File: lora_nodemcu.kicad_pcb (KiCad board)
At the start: 4 copper layers, 33 x 39.4 mm, 9 parts, among them U1 RFM95, U3 WeMos_mini

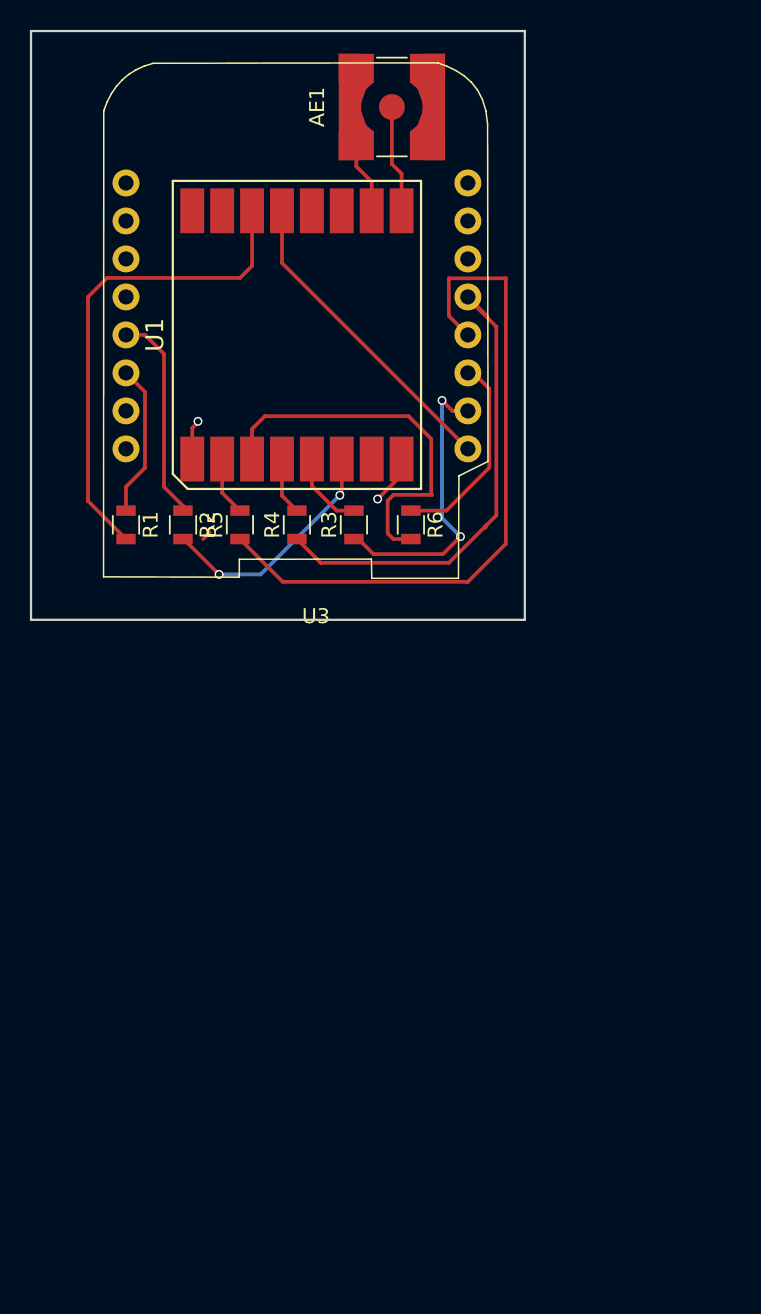
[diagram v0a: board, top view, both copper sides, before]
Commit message: Relayed out board.
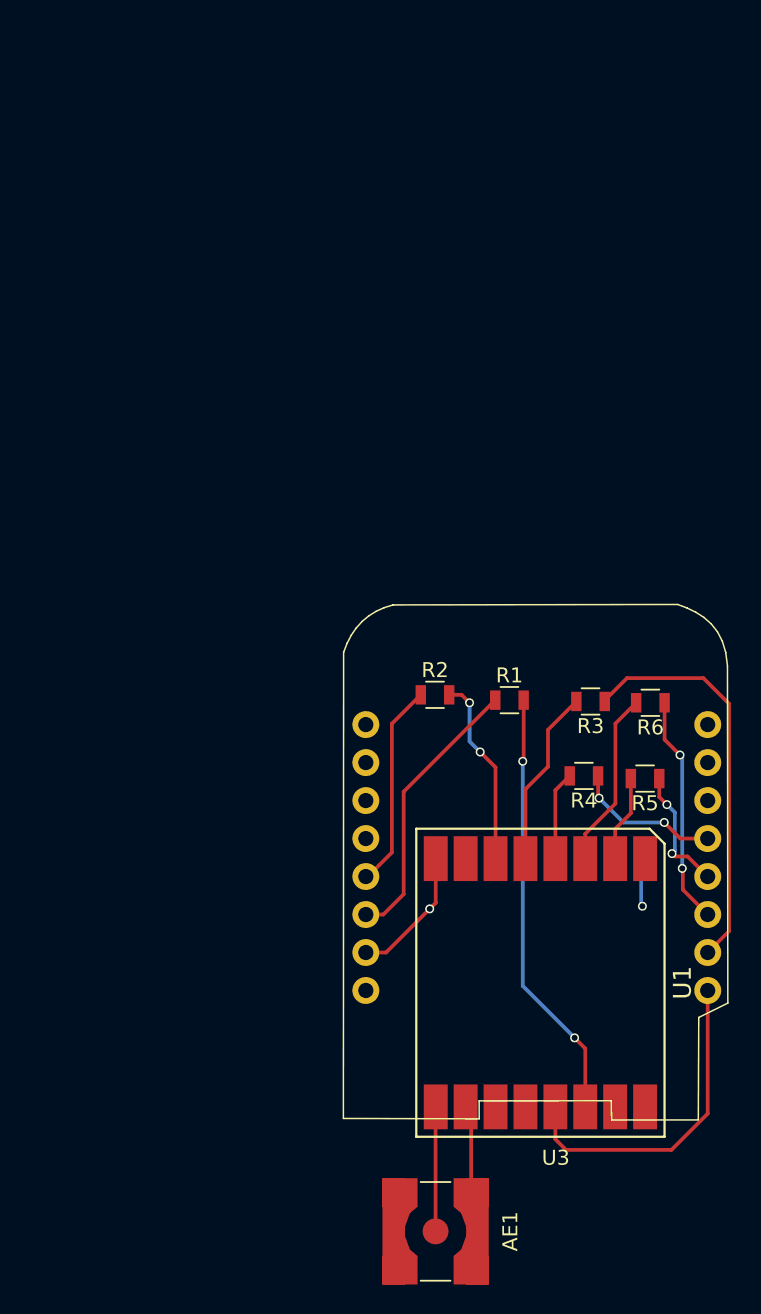
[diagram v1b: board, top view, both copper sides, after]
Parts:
- AE1: value Ant -> Antenna_Shield
- moved AE1 75.2 mm to (156.6, 150.1), turned to 270 degrees
- moved U1 46.3 mm to (163.6, 133.5), turned to 180 degrees
- moved U3 39.6 mm to (163.4, 126.4)
- moved R5 32.0 mm to (170.6, 119.8), turned to 180 degrees
- moved R1 28.2 mm to (161.5, 114.6), turned to 0 degrees
- moved R4 25.5 mm to (166.5, 119.7), turned to 180 degrees
- moved R2 20.3 mm to (156.6, 114.2), turned to 0 degrees
- moved R6 20.0 mm to (171.0, 114.8), turned to 180 degrees
- moved R3 19.7 mm to (167.0, 114.7), turned to 180 degrees
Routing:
- net /MISO: track 45.9 -> 8.55 mm, vias 0 -> 2
- net /SCK: track 32.8 -> 9.89 mm, vias 0 -> 2
- net Net-(R6-Pad2): track 25.7 -> 11.8 mm
- net Net-(R1-Pad1): track 10.3 -> 18.6 mm
- net Net-(AE1-Pad2): track 19.0 -> 11.1 mm
- net /SS: track 19.7 -> 26.9 mm, vias 2 -> 0
- net Net-(R3-Pad2): track 5.29 -> 11.9 mm
- net Net-(R1-Pad2): track 32.8 -> 29.0 mm, vias 0 -> 2
- net Net-(R2-Pad2): track 16.1 -> 12.7 mm
- net GND: track 6.02 -> 9.01 mm, vias 2 -> 1
- net (no net): track 0.63 -> 2.97 mm, vias 0 -> 1
- net Net-(R4-Pad2): track 3.86 -> 5.93 mm
- net Net-(R5-Pad2): track 3.94 -> 5.79 mm
- net /MOSI: track 13.6 -> 15.4 mm, vias 0 -> 2
- net Net-(AE1-Pad1): track 7.21 -> 8.33 mm
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- removed copper zone on In1.Cu, net GND
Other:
- board outline removed
